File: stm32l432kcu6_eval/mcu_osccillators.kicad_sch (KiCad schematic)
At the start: 9 parts, among them U1 STM32L432KCUx, Y1 ASFL1-40.000MHZ-EC-T, Y2 FC-135_32.7680KA-A3_12_5_pF

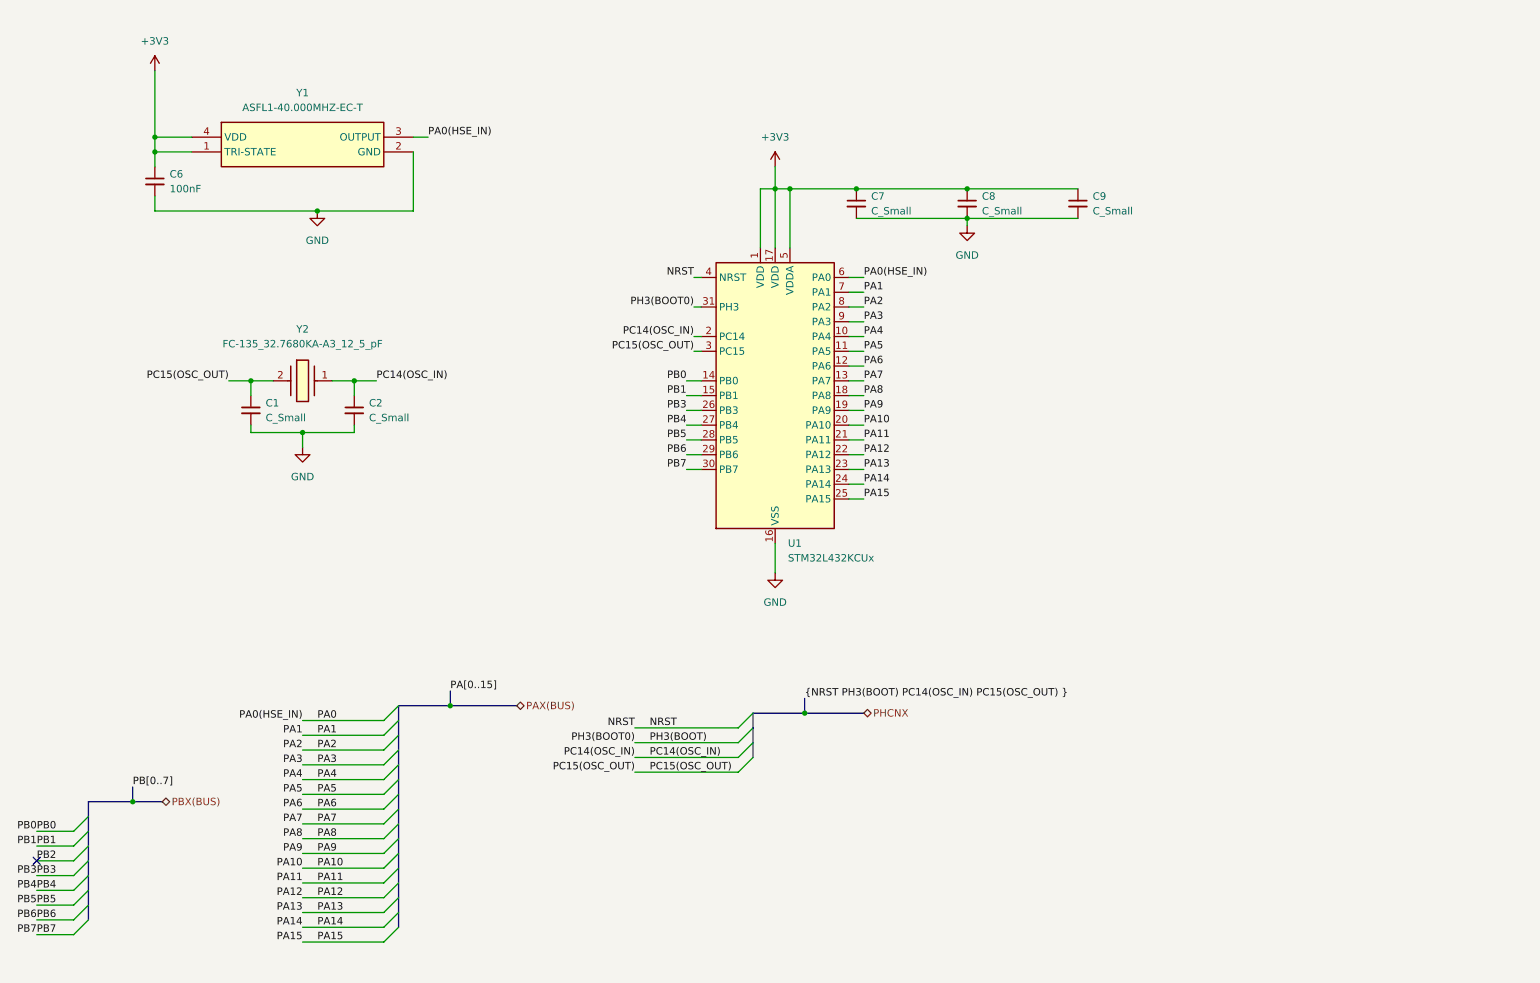
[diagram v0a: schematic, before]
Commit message: organisation save 1
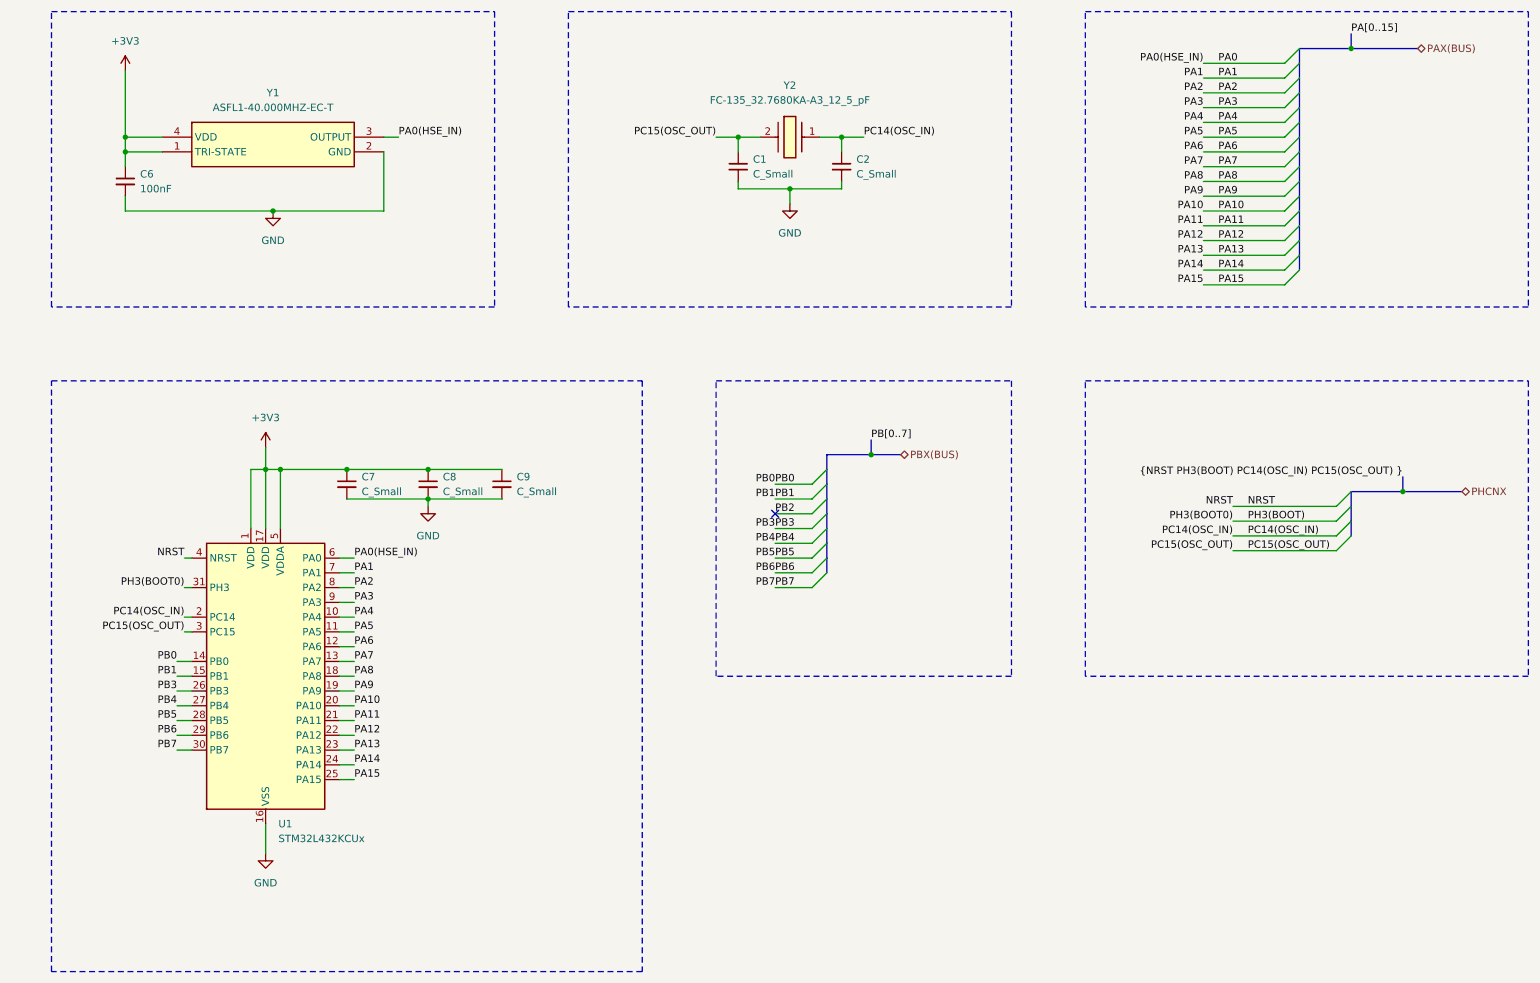
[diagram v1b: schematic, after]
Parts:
- C1, C2: footprint Capacitor_SMD:C_0603_1608Metric -> Capacitor_SMD:C_0402_1005Metric
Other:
- moved on the sheet: C1, C2, C6, C7, C8, C9, U1, Y1, Y2
